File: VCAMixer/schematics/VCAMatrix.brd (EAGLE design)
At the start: 119.8 x 101.3 mm, 290 parts, among them IC1 QUAD_OPAMPD, IC2 TL074D, IC4 TL072D, Q1 BC846ALT1SMD, Q10 BSS123, Q2 BC846ALT1SMD, Q3 BC846ALT1SMD, Q4 BC846ALT1SMD, Q5 BC846ALT1SMD, Q6 BC846ALT1SMD, Q7 BC846ALT1SMD, Q8 BC846ALT1SMD, Q9 BSS84, X1 53048-05, X2 53048-05

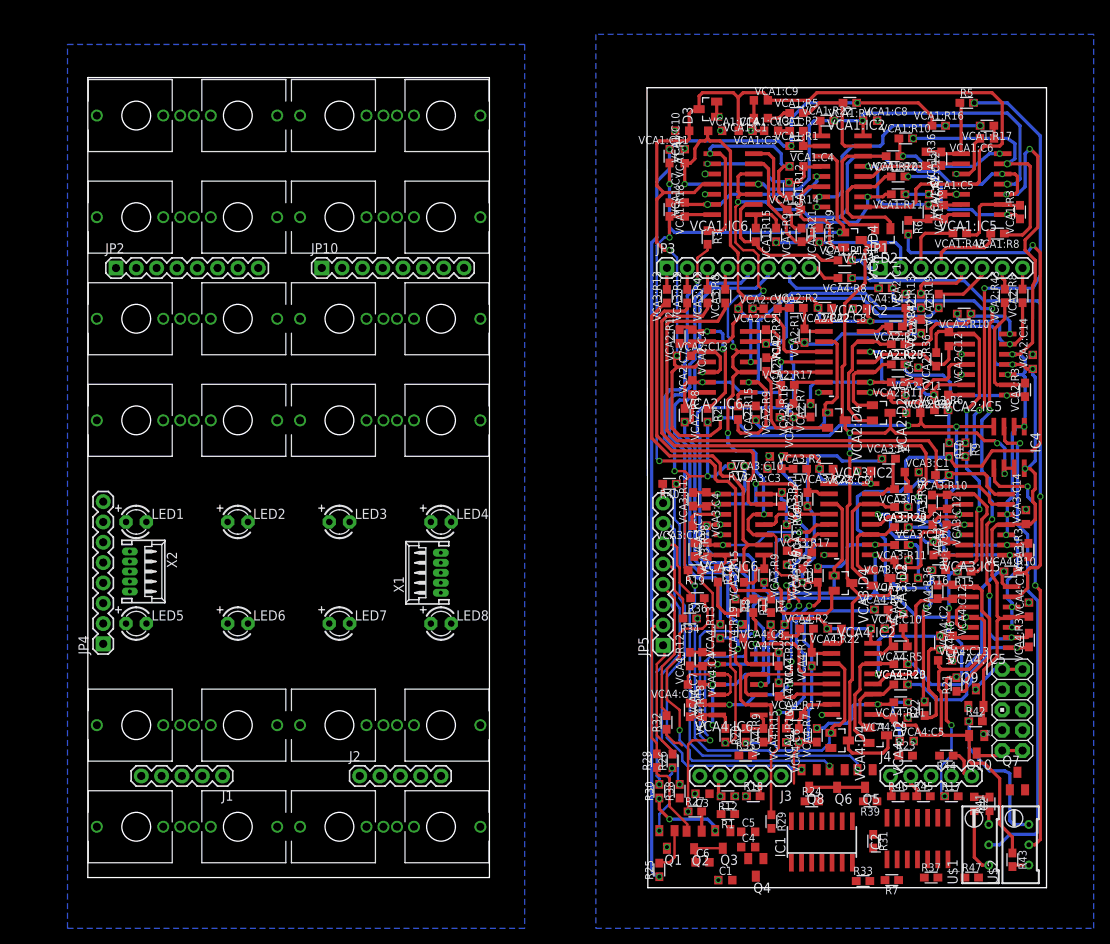
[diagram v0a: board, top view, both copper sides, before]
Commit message: Latest Update To VCA Board
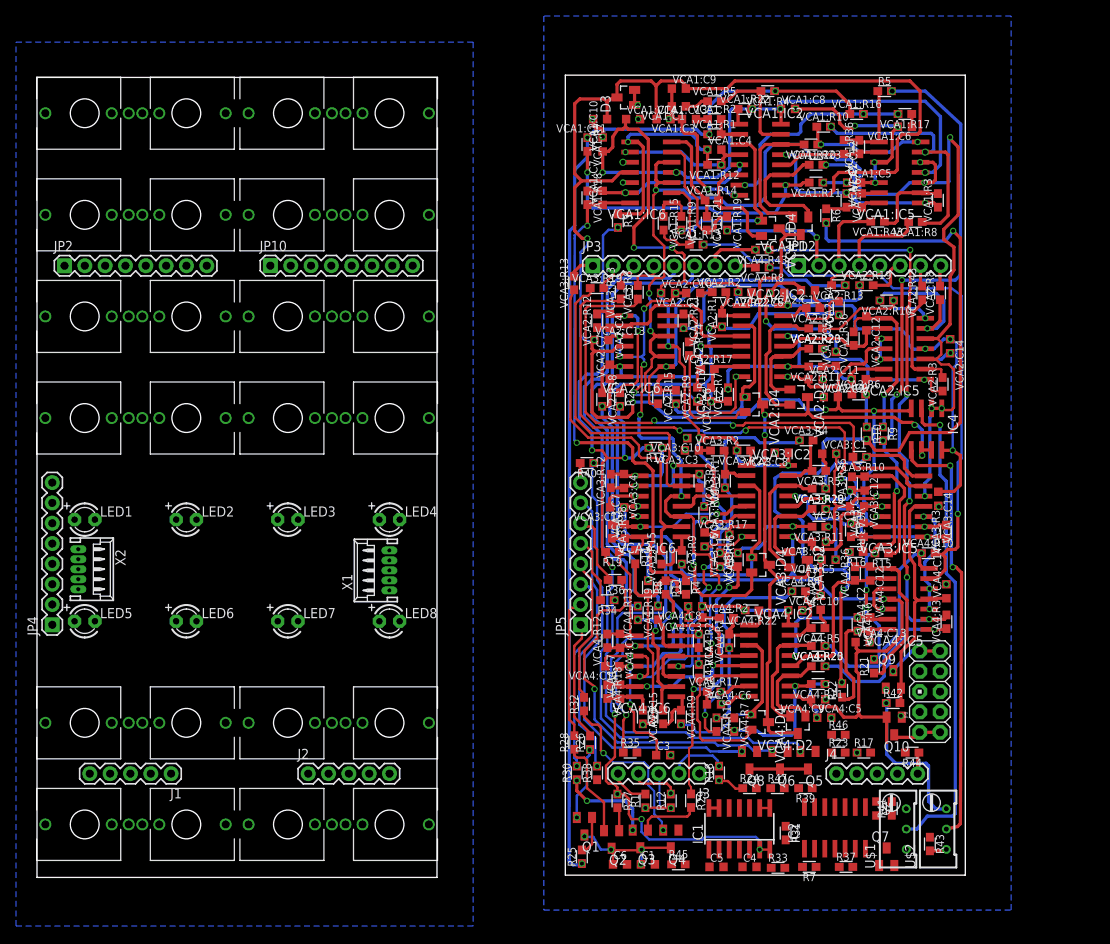
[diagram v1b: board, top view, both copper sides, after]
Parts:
- moved R45 31.8 mm to (73.8, 1.65)
- moved R47 26.7 mm to (86.2, 11.2)
- moved Q7 18.9 mm to (99.9, 2.60)
- moved VCA1:R13 18.7 mm to (76.0, 79.1)
- moved VCA4:R43 16.1 mm to (84.3, 78.5)
- moved R35 14.4 mm to (67.8, 15.6)
- moved VCA4:R15 12.7 mm to (71.9, 20.1), turned to 90 degrees
- moved VCA2:C1 12.3 mm to (90.0, 73.4), turned to 180 degrees
- moved R17 12.2 mm to (97.0, 15.6)
- moved C2 12.2 mm to (98.6, 8.63)
- moved R41 12.2 mm to (100.5, 8.63)
- moved VCA1:R21 11.9 mm to (77.4, 81.8)
- moved VCA1:R9 11.9 mm to (74.2, 81.8)
- moved VCA3:R13 11.7 mm to (60.8, 74.3)
- moved VCA1:R15 11.6 mm to (72.0, 81.8)
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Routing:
- net GND: track 83.5 -> 225.9 mm, vias 52 -> 62
- net +12V: track 290.9 -> 317.8 mm, vias 24 -> 28
- net N$3: track 104.1 -> 130.2 mm, vias 6 -> 8
- net N$60: track 3.21 -> 21.7 mm, vias 0 -> 2
- net N$11: track 106.9 -> 90.4 mm, vias 11 -> 10
- net VCA4:N$7: track 7.20 -> 22.0 mm
- net CV_AA: track 3.99 -> 13.0 mm
- net VCA4:IC2_4: track 62.2 -> 71.1 mm
- net N$51: track 0.00 -> 7.67 mm
- net CV_DC: track 13.1 -> 6.67 mm
- net VCA1:IC2_5: track 19.7 -> 13.6 mm
- net N$24: track 52.2 -> 57.6 mm
- net OUTPUT_B: track 21.0 -> 26.3 mm, vias 1 -> 2
- net N$22: track 33.7 -> 28.4 mm
- net IN_A: track 0.00 -> 4.98 mm
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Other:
- board size 119.8 x 101.3 mm -> 116 x 100.3 mm
